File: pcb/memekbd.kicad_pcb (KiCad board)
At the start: 2 copper layers, 134.1 x 130.9 mm, 207 parts, among them J1 AudioJack4, J2 AudioJack4, SW1 SW_Push, SW10 SW_Push, SW11 SW_Push, SW12 SW_Push, SW13 SW_Push, SW14 SW_Push, SW15 SW_Push, SW16 SW_Push, SW17 SW_Push, SW18 SW_Push, SW19 SW_Push, SW2 SW_Push, SW20 SW_Push, SW21 SW_Push, SW22 SW_Push, SW23 SW_Push, SW24 SW_Push, SW25 SW_Push, SW26 SW_Push, SW27 SW_Push, SW28 SW_Push, SW29 SW_Push, SW3 SW_Push, SW30 SW_Push, SW31 SW_Push, SW32 SW_Push, SW33 SW_Push, SW34 SW_Push, SW35 SW_Push, SW36 SW_Push, SW37 SW_Push, SW38 SW_Push, SW39 SW_Push, SW4 SW_Push, SW40 SW_Push, SW41 SW_Push, SW42 SW_Push, SW43 SW_Push, SW44 SW_Push, SW45 SW_Push, SW46 SW_Push, SW47 SW_Push, SW48 SW_Push, SW5 SW_Push, SW6 SW_Push, SW7 SW_Push, SW8 SW_Push, SW9 SW_Push, U1 ProMicro, U2 ProMicro

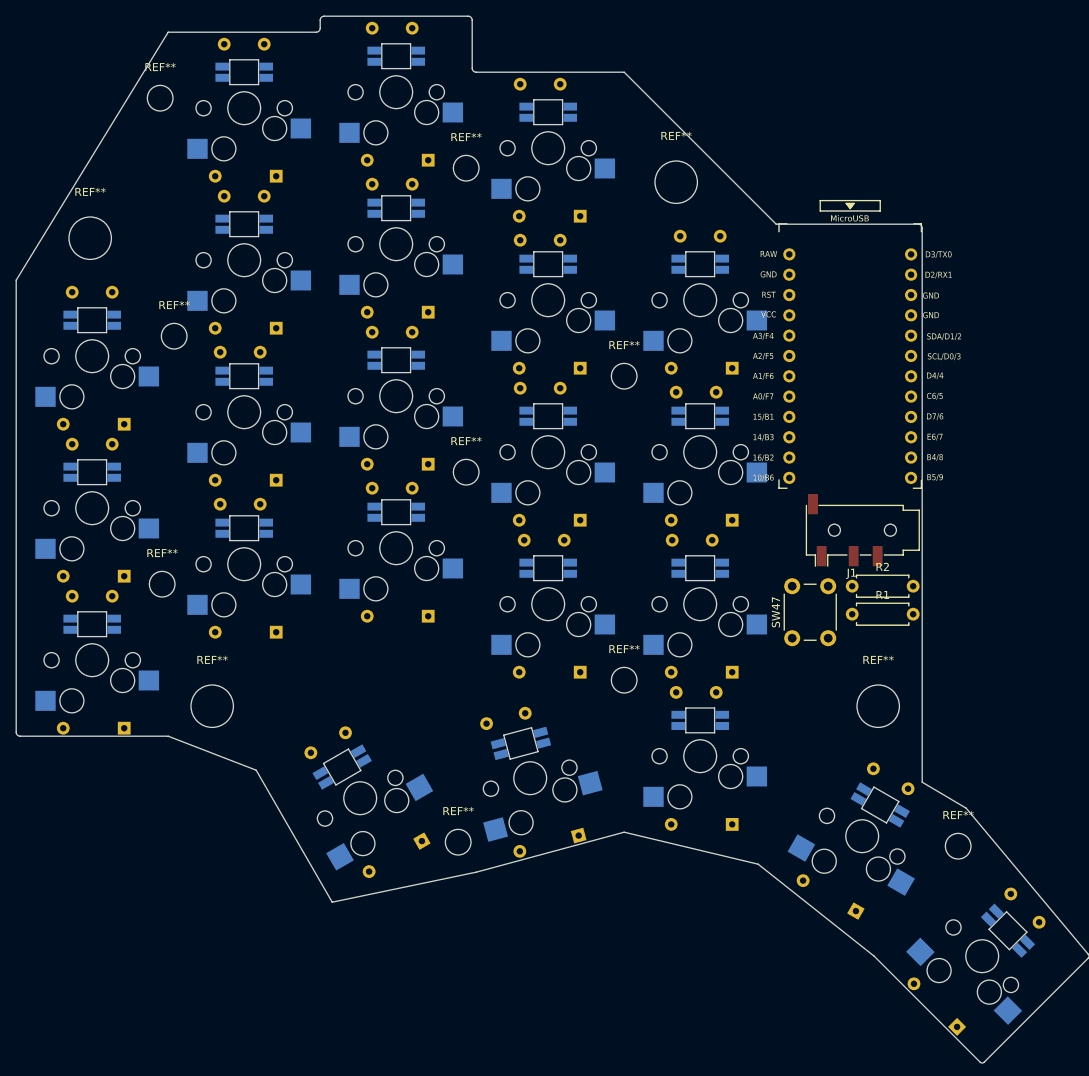
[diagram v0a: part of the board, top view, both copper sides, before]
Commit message: Some routing
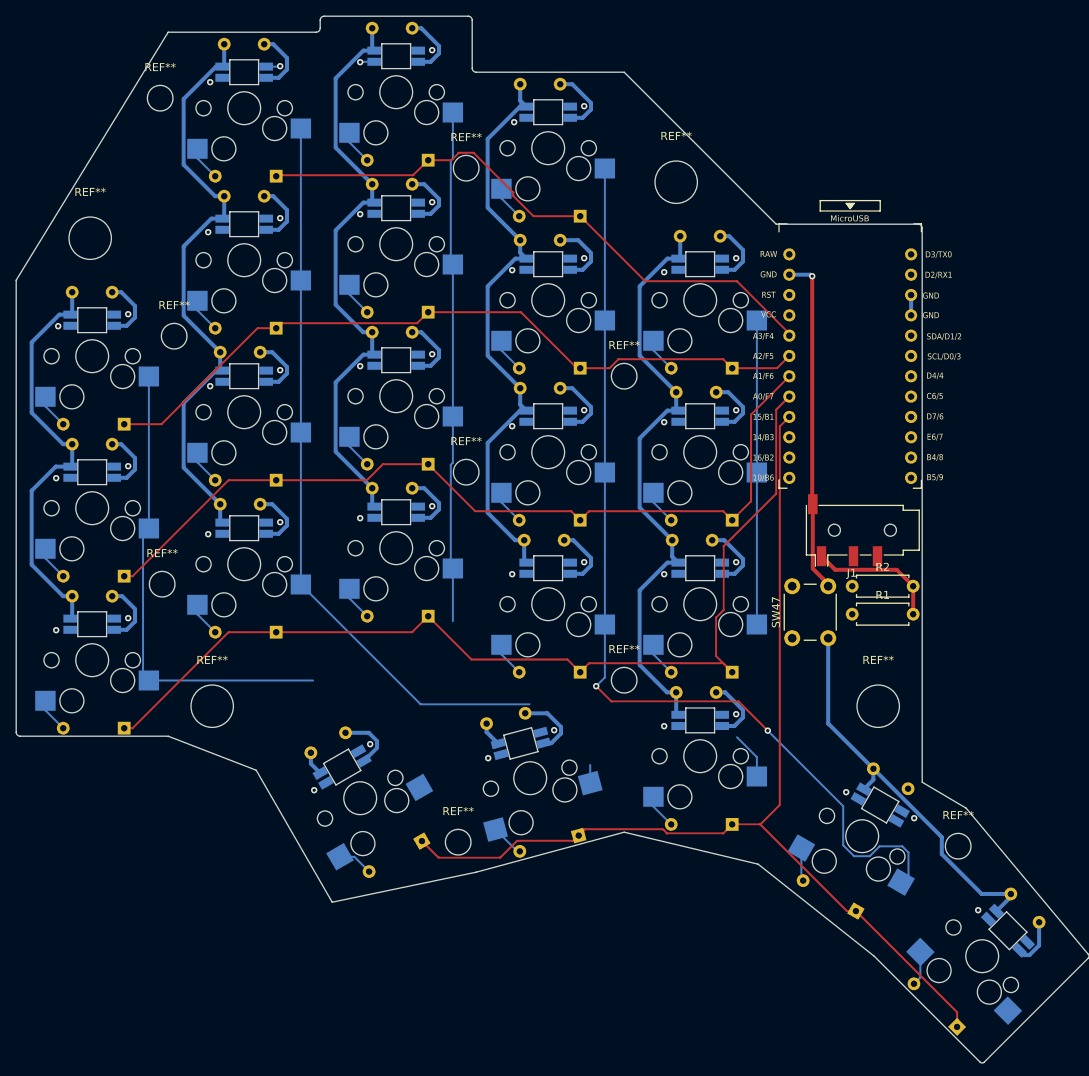
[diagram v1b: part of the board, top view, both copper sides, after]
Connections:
- J1 pad R1: /lSCL -> /lSDA
- J1 pad R2: /lSDA -> /lSCL
- J2 pad R1: /rSCL -> /rSDA
- J2 pad R2: /rSDA -> /rSCL
- R1 pad 1: /lSDA -> /lSCL
- R2 pad 1: /lSCL -> /lSDA
- R3 pad 1: /rSDA -> /rSCL
- R4 pad 1: /rSCL -> /rSDA
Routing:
- net GND: track 0.00 -> 452.3 mm, vias 0 -> 1
- net +5V: track 0.00 -> 194.4 mm
- net /lrow4: track 0.00 -> 133.9 mm
- net /lrow3: track 0.00 -> 124.7 mm
- net /lcol3: track 0.00 -> 121.1 mm, vias 0 -> 2
- net /lrow2: track 0.00 -> 106.6 mm
- net /lcol1: track 0.00 -> 94.1 mm
- net /lrow1: track 0.00 -> 93.4 mm
- net /lrow0: track 0.00 -> 75.2 mm
- net /lcol2: track 0.00 -> 70.0 mm
- net /lcol0: track 0.00 -> 59.2 mm
- net /lcol4: track 0.00 -> 38.0 mm
- net Net-(D4-Pad2): track 0.00 -> 4.40 mm
- net Net-(D14-Pad2): track 0.00 -> 4.36 mm
- net Net-(D8-Pad2): track 0.00 -> 4.34 mm
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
